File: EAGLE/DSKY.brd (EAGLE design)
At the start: 100 x 80 mm, 6 parts, among them IC1 74LS595N, IC2 74LS595N, IC3 74LS595N

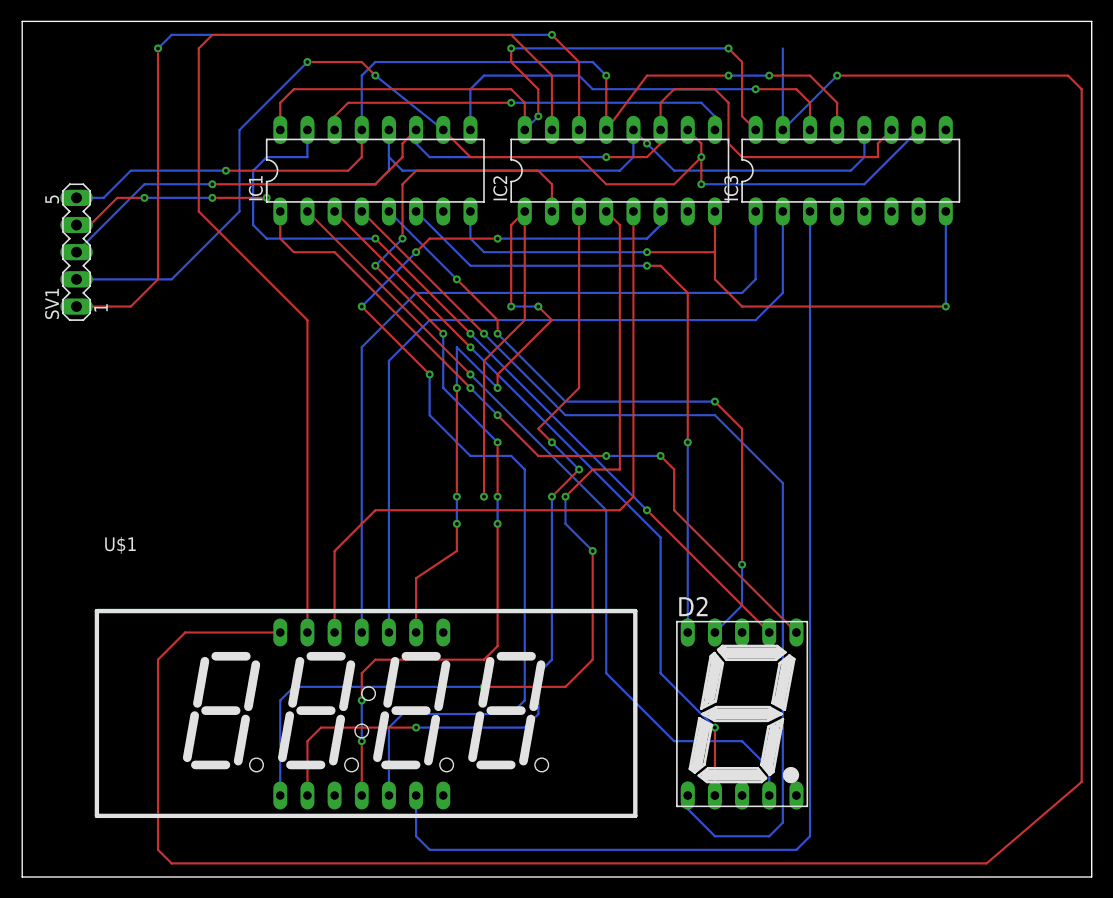
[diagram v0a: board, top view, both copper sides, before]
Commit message: Update BRD
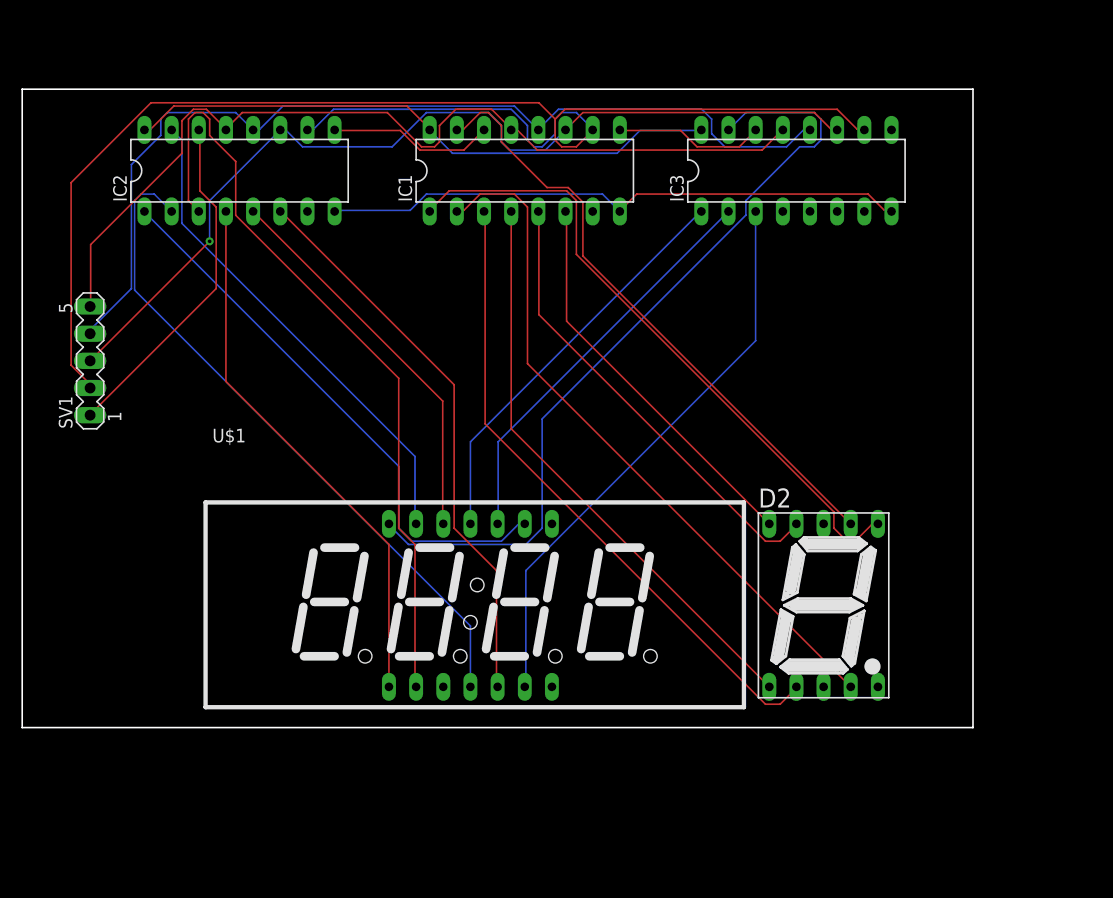
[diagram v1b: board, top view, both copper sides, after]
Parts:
- moved IC2 35.6 mm to (20.3, 66.0)
- moved U$1 14.4 mm to (36.8, 29.2)
- moved IC1 14.0 mm to (47.0, 66.0)
- moved D2 12.7 mm to (74.9, 25.4)
- moved SV1 10.2 mm to (6.35, 48.3)
- moved IC3 5.08 mm to (72.4, 66.0)
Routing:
- net N$15: track 222.9 -> 75.2 mm, vias 1 -> 0
- net N$1: track 99.0 -> 46.3 mm
- net N$18: track 100.1 -> 53.4 mm
- net N$25: track 77.6 -> 32.2 mm, vias 2 -> 0
- net N$7: track 97.8 -> 52.9 mm, vias 4 -> 0
- net N$12: track 93.4 -> 54.4 mm, vias 1 -> 0
- net N$5: track 86.8 -> 50.8 mm, vias 3 -> 0
- net N$17: track 72.5 -> 38.2 mm
- net N$16: track 72.5 -> 38.2 mm
- net N$24: track 104.8 -> 138.1 mm, vias 4 -> 0
- net N$3: track 91.7 -> 62.9 mm, vias 8 -> 0
- net N$26: track 28.2 -> 0.00 mm, vias 1 -> 0
- net N$6: track 64.3 -> 36.6 mm
- net N$21: track 39.7 -> 14.0 mm, vias 1 -> 0
- net N$20: track 39.2 -> 15.5 mm, vias 1 -> 0
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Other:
- board size 100 x 80 mm -> 88.9 x 59.7 mm
